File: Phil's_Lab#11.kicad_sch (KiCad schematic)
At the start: 50 parts, among them J1 Screw_Terminal_01x02, J2 SWD, J3 Conn_01x04, J4 Conn_01x04, J5 USB_B_Micro, Q1 AO3401A, SW1 SW_SPDT, U1 STM32F405RGT6, U3 USBLC6-2SC6, Y1 16MHz

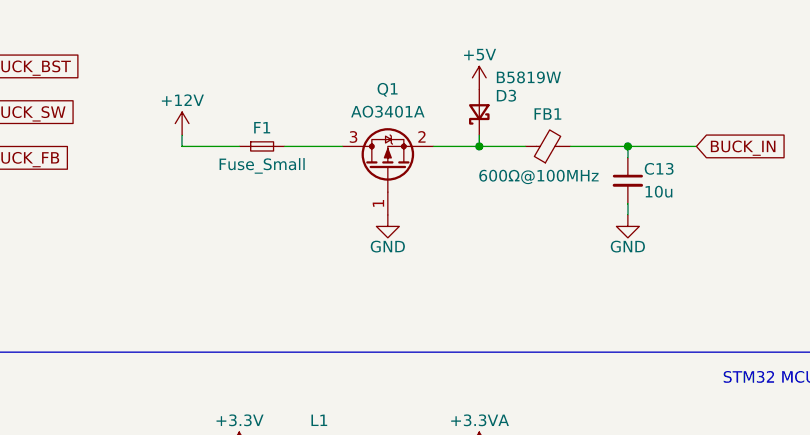
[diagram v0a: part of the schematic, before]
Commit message: .
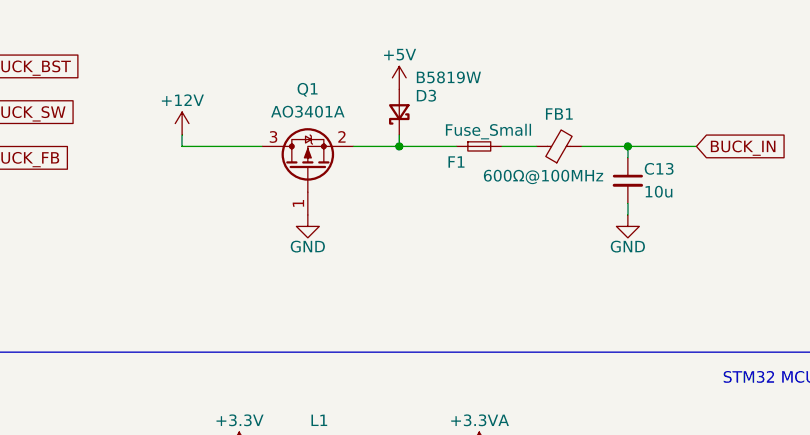
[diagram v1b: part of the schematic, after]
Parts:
- U2: value ~ -> (none)
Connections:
- net +12V: now also Q1.3 (D); no longer F1.1
- net at D3.1 (K), Q1.2 (S): now also F1.1; no longer FB1.1
- net at F1.2: now also FB1.1; no longer Q1.3 (D)
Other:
- moved on the sheet: D3, F1, FB1, Q1

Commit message: .
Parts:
- J5: footprint Connector_USB:USB_Micro-AB_Molex_47590-0001 -> Connector_USB:USB_Micro-B_Amphenol_10118193-0001LF_Horizontal
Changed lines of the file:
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@@
 			)
 		)
-		(property "Footprint" "Connector_USB:USB_Micro-AB_Molex_47590-0001"
+		(property "Footprint" "Connector_USB:USB_Micro-B_Amphenol_10118193-0001LF_Horizontal"
 			(at 194.31 146.05 0)
 			(hide yes)

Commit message: .
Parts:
- C1, C2: LCSC Part # (none) -> C23630
- C10: LCSC Part # (none) -> C15195
- C11, C12: LCSC Part # (none) -> C346183
- C13, C15, C16: LCSC Part # (none) -> C13585
- C14: LCSC Part # (none) -> C1846
- C3: LCSC Part # (none) -> C19666
- C4, C5, C6, C7, C8: LCSC Part # (none) -> C1525
- C9: LCSC Part # (none) -> C52923
- D2, D3: LCSC Part # (none) -> C9900270134
- FB1: LCSC Part # (none) -> C1002
- H1, H2, H3, H4: now in the parts list
- J2: footprint Connector_PinSocket_1.27mm:PinSocket_2x05_P1.27mm_Vertical_SMD -> Connector_PinHeader_1.27mm:PinHeader_2x05_P1.27mm_Vertical_SMD
- L1: LCSC Part # (none) -> C26443
- L2: LCSC Part # (none) -> C139506
- Q1: LCSC Part # (none) -> C15127
- R1: LCSC Part # (none) -> C25744
- R10, R9: LCSC Part # (none) -> C25879
- R11: LCSC Part # (none) -> C22843
- R12: LCSC Part # (none) -> C21190
- R2: LCSC Part # (none) -> C23231
- R4, R5: LCSC Part # (none) -> C25803
- R6: LCSC Part # (none) -> C22809
- R7: LCSC Part # (none) -> C22966
- R8: LCSC Part # (none) -> C25819
- SW1: LCSC Part # (none) -> C22449121
- U1: LCSC Part # (none) -> C15742
- U2: LCSC Part # (none) -> C14259
- U3: LCSC Part # (none) -> C558442
- Y1: LCSC Part # (none) -> C2905353
